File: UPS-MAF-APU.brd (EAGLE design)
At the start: 65 x 56 mm, 35 parts, among them J1 CONNECTOR_PI_40_PIN, J2 Barrel DC In, J3 OLED, J4 OSTOQ045451, J5 External DS18B20 Temp, J6 FTDI Serial Console, J7 MagJack, U1 OLED_I2C, U2 SI7006-A20-IM, U4 INA260AIPW, U6 ENC28J60_SS, U7 5V SMPS, Y1 ECS-250-20-3X-EN-TR

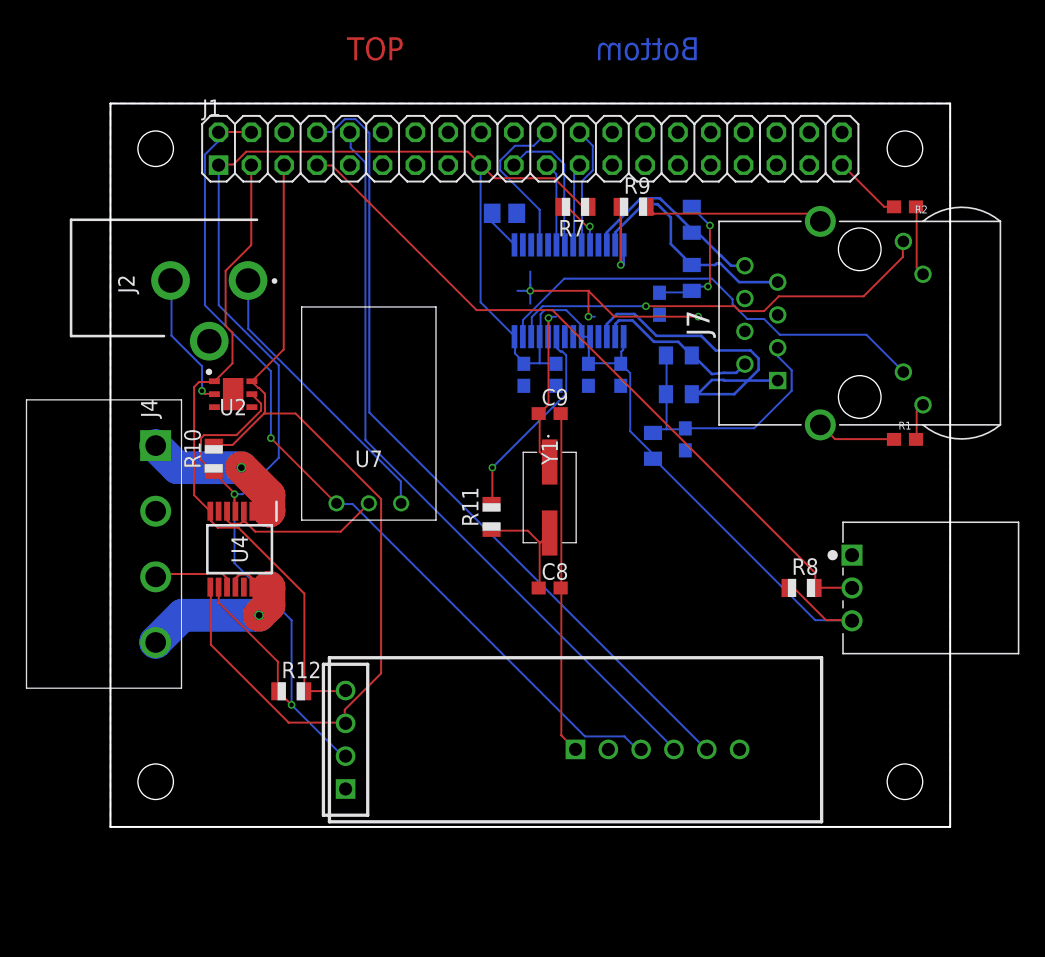
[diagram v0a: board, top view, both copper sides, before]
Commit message: README
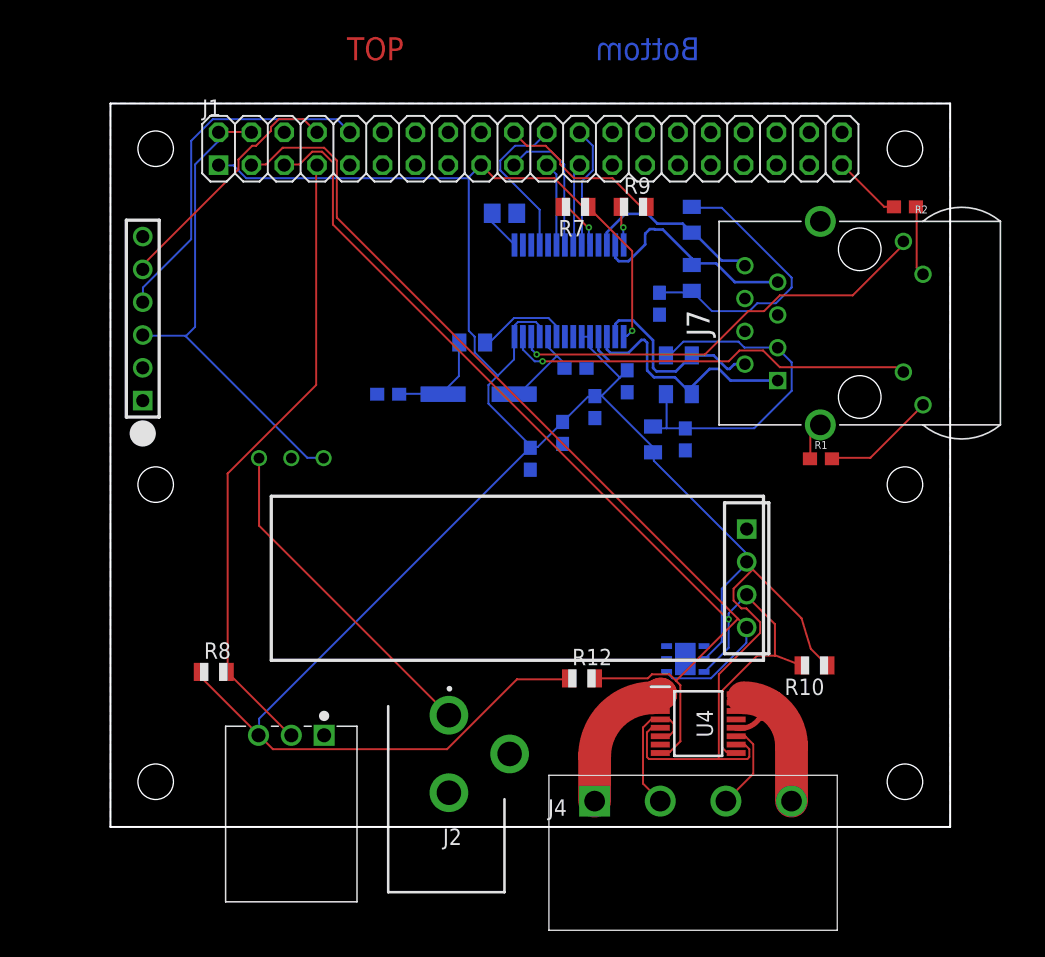
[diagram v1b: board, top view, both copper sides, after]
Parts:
- moved J5 52.5 mm to (14.0, 1.00), turned to 0 degrees
- moved R10 49.2 mm to (54.5, 12.5), turned to 180 degrees
- moved R8 46.0 mm to (8.00, 12.0)
- moved J4 43.7 mm to (37.5, 2.00), turned to 0 degrees
- moved J6 43.0 mm to (2.50, 33.0), flipped to the top, turned to 90 degrees
- moved U2 40.6 mm to (44.5, 13.0), flipped to the bottom, turned to 180 degrees
- moved J2 39.6 mm to (30.5, 5.65), turned to 180 degrees
- moved U4 38.0 mm to (45.5, 8.00), turned to 0 degrees
- moved J3 33.5 mm to (49.2, 19.2), turned to 270 degrees
- moved R12 22.5 mm to (36.5, 11.5)
- moved C8 19.5 mm to (21.5, 33.5), flipped to the bottom
- moved R11 13.6 mm to (28.0, 37.5), flipped to the bottom, turned to 180 degrees
- moved U1 13.3 mm to (31.5, 19.2), turned to 180 degrees
- moved Y1 9.71 mm to (28.5, 33.5), flipped to the bottom, turned to 0 degrees
- moved U7 6.95 mm to (14.0, 35.5), flipped to the bottom
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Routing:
- net TX_OR: track 63.5 -> 19.5 mm
- net 3.3V: track 179.7 -> 221.5 mm, vias 2 -> 1
- net GND: track 83.0 -> 43.2 mm, vias 1 -> 0
- net SDA: track 51.4 -> 86.6 mm
- net RX_OT: track 58.2 -> 27.4 mm
- net 5V: track 67.5 -> 37.4 mm, vias 1 -> 0
- net N$8: track 21.3 -> 0.00 mm, vias 3 -> 0
- net N$6: track 10.8 -> 22.5 mm, vias 2 -> 0
- net TPOUT_P: track 28.4 -> 19.2 mm
- net OOUT: track 15.8 -> 7.41 mm, vias 1 -> 0
- net N$4: track 55.7 -> 49.2 mm
- net OIN: track 13.9 -> 7.53 mm, vias 1 -> 0
- net N$1: track 21.7 -> 27.7 mm
- net N$7: track 2.91 -> 8.83 mm
- net SCK: track 73.5 -> 78.8 mm, vias 0 -> 1
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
